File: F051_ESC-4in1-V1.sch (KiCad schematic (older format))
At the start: 45 parts, among them J1 Conn_01x02, J10 Conn_01x03, J11 Conn_01x03, J12 Conn_01x04, J13 Conn_01x03, J14 Conn_01x03, J15 Conn_01x04, J16 Conn_01x03, J17 Conn_01x03, J2 Conn_01x10, J3 Conn_01x04, J4 Conn_01x03, J5 Conn_01x04, J6 Conn_01x03, J7 Conn_01x03, J8 Conn_01x03, J9 Conn_01x04

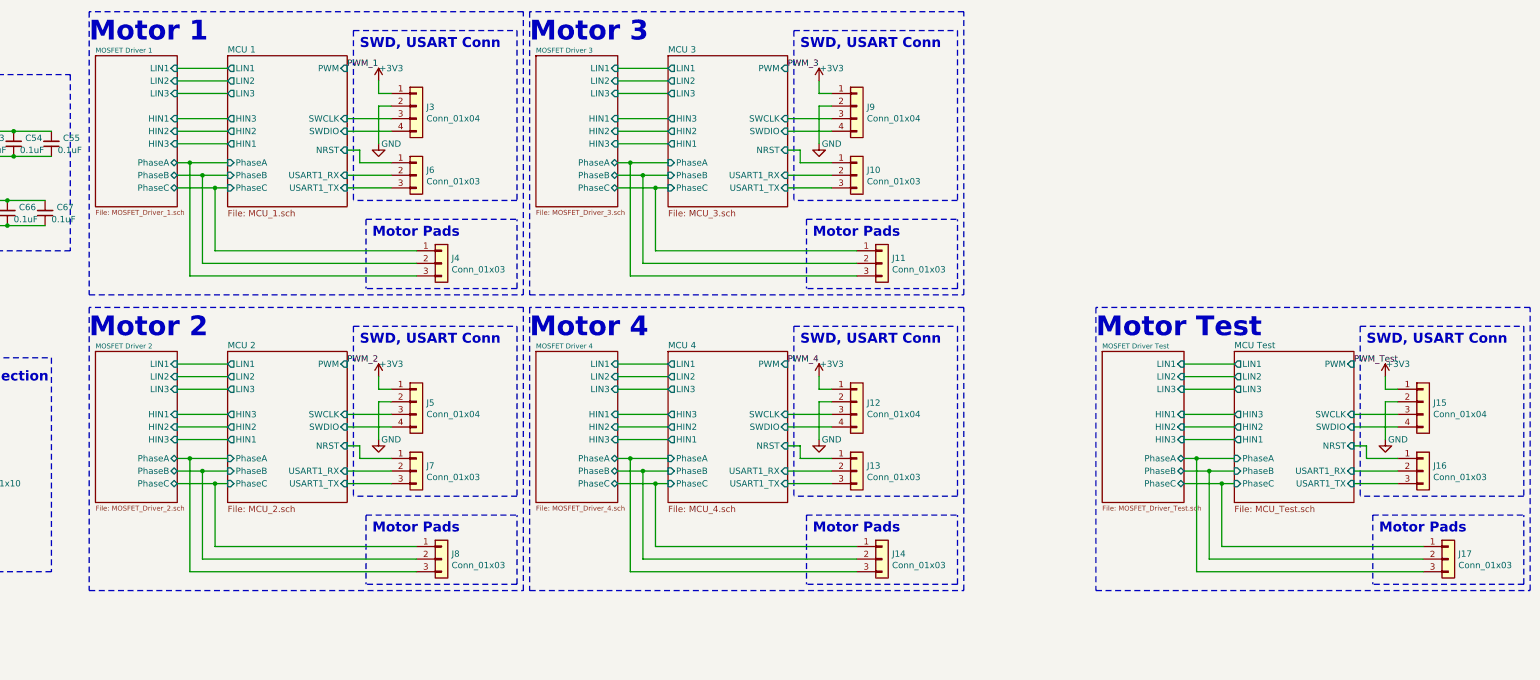
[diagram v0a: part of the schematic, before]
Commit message: More design changes
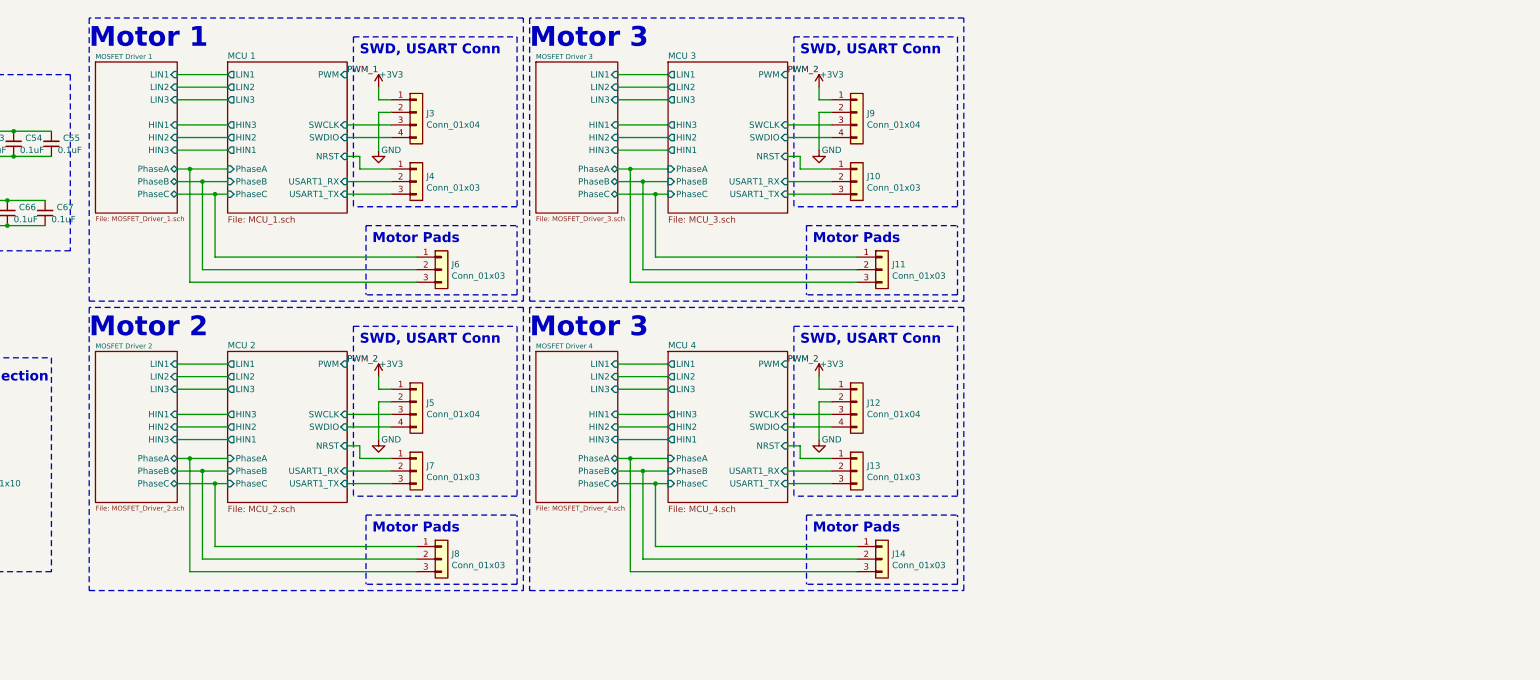
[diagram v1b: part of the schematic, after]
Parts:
- removed J15: Conn_01x04, Connector_PinHeader_2.54mm:PinHeader_1x04_P2.54mm_Vertical, symbol Connector_Generic:Conn_01x04
- removed J16: Conn_01x03, Connector_PinHeader_2.54mm:PinHeader_1x03_P2.54mm_Vertical, symbol Connector_Generic:Conn_01x03
- removed J17: Conn_01x03, Connector_Wire:Conn_MotorPhase, symbol Connector_Generic:Conn_01x03
- J4: footprint Connector_Wire:Conn_MotorPhase -> Connector_PinHeader_2.54mm:PinHeader_1x03_P2.54mm_Vertical
- J6: footprint Connector_PinHeader_2.54mm:PinHeader_1x03_P2.54mm_Vertical -> Connector_Wire:Conn_MotorPhase
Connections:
- net MCU 1/NRST: now also J4.1 (Pin_1); no longer J6.1 (Pin_1)
- net MCU 1/PhaseA: now also J6.3 (Pin_3); no longer J4.3 (Pin_3)
- net MCU 1/PhaseB: now also J6.2 (Pin_2); no longer J4.2 (Pin_2)
- net MCU 1/PhaseC: now also J6.1 (Pin_1); no longer J4.1 (Pin_1)
- net MCU 1/USART1_RX: now also J4.2 (Pin_2); no longer J6.2 (Pin_2)
- net MCU 1/USART1_TX: now also J4.3 (Pin_3); no longer J6.3 (Pin_3)
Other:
- note removed: "Motor 4"
- note removed: "Motor Test"
